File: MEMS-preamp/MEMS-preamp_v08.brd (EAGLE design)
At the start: 51 x 30 mm, 46 parts, among them IC1 DMN2400, IC2 BQ21040, IC3 BQ297X, IC4 SC4503, IC5 TPS7A49, IC6 OPA2134, J2 Battery, SW1 SPDT

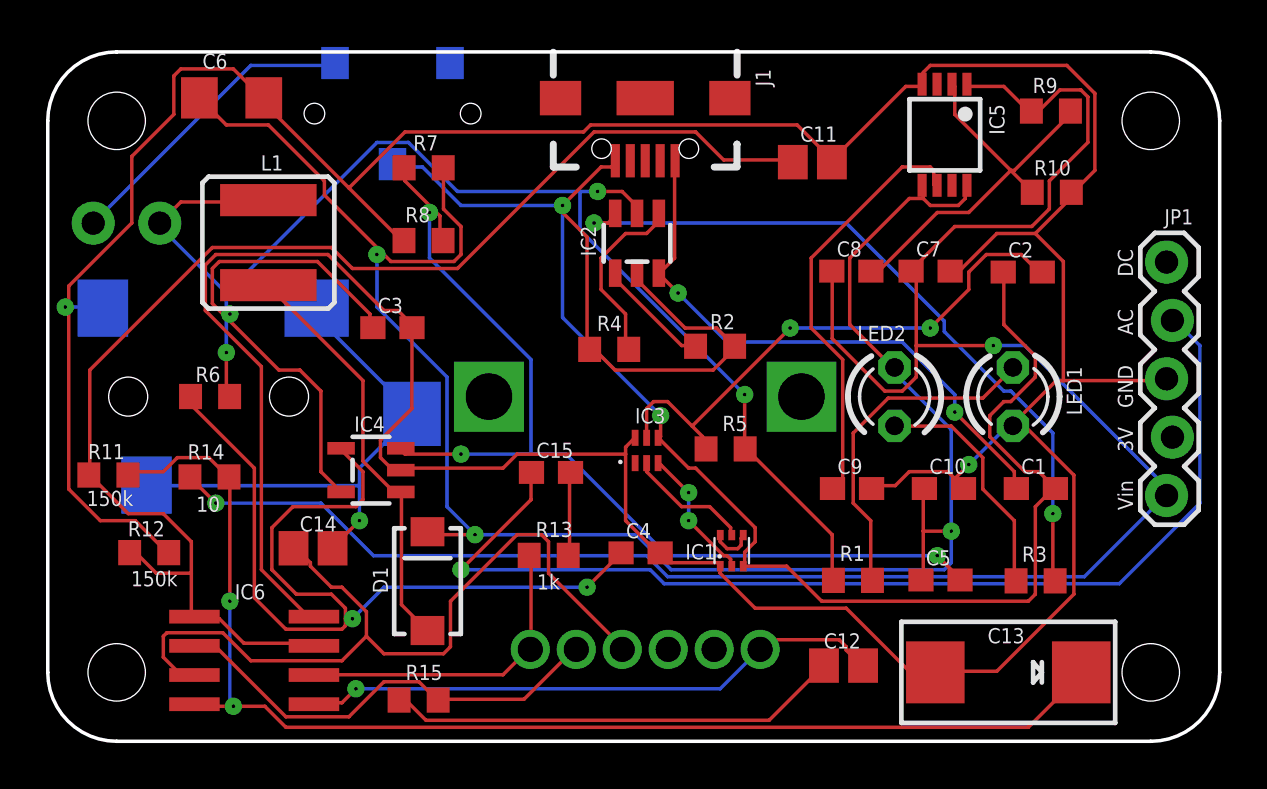
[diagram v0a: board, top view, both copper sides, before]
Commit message: Add files via upload
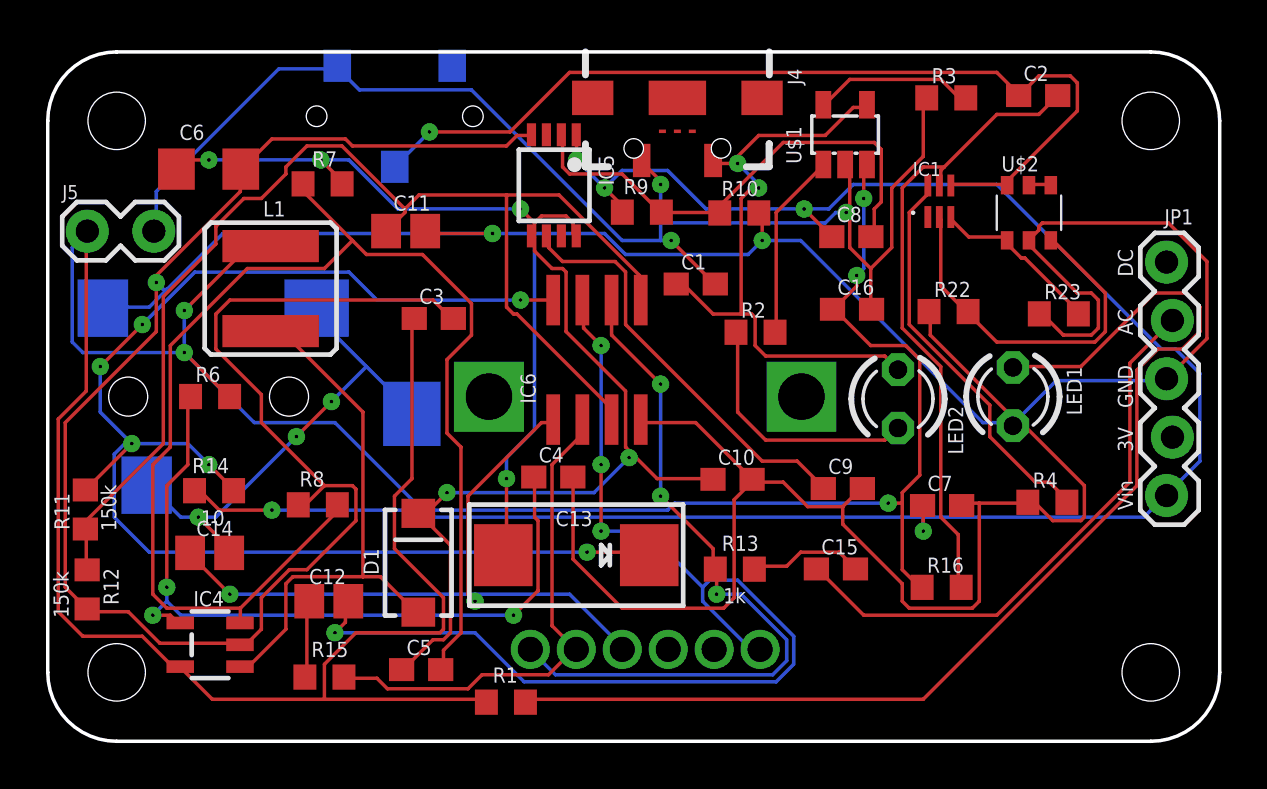
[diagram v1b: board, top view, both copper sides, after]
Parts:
- removed IC2: BQ21040, CMU-ArtFab:SOT23-6
- removed IC3: BQ297X, CMU-ArtFab:WSON-6
- removed J1: (no value), SparkFun-Connectors:USB-B-MICRO-SMD_RED_PASTE
- removed J2: Battery, SparkFun-Connectors:1X02_LOCK
- removed R5: 330, CMU-ArtFab:R0603
- removed SW1: SPDT, CMU-ArtFab:SWITCH_SPDT_CL-SB-12B
- added C16: 4.7uF, rcl:C0603
- added J4: (no value), CMU-ArtFab:USB-B-MICRO-SMD_RED_PASTE
- added J5: Battery, SparkFun-Connectors:1X02_LOCK
- added R16: 330, CMU-ArtFab:R0603
- added R22, R23: 10M, CMU-ArtFab:R0603
- added SW3: SPDT, CMU-ArtFab:SWITCH_SPDT_CL-SB-12B
- added U$1: MCP73831, CMU-ArtFab:SOT-23-5
- added U$2: QS6K1, CMU-ArtFab:SOT457R_PHILIPS
- C1: value 10uF -> 4.7uF
- IC1: value DMN2400 -> BQ297X; device CMU-ArtFab:SOT-563 -> CMU-ArtFab:WSON-6-LONG
- IC6: value OPA2134 -> TL072D
- LED2: value (none) -> Charge
- R2: value 10k -> 470
- R3: value 1k -> 5k
- R4: value 10k -> 2.2k
- moved C5 22.9 mm to (16.2, 3.12)
- moved C12 22.6 mm to (12.2, 6.09)
- moved R3 21.4 mm to (39.1, 28.0)
- moved R4 20.2 mm to (43.5, 10.4)
- moved IC6 19.8 mm to (23.9, 16.6), turned to 0 degrees
- moved C13 19.5 mm to (23.0, 8.10)
- moved R9 18.3 mm to (25.9, 23.0)
- moved C11 18.0 mm to (15.6, 22.2)
- moved IC1 17.7 mm to (38.8, 23.5)
- moved C1 17.3 mm to (28.2, 19.9)
- moved IC5 17.1 mm to (22.0, 24.2)
- moved R1 16.0 mm to (19.9, 1.70)
- moved R10 13.6 mm to (30.1, 23.0)
- moved C15 13.1 mm to (34.3, 7.50)
- moved R8 12.4 mm to (11.8, 10.3)
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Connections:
- removed net GND2: C1.2, C2.1, IC1.3, IC2.5, IC3.4, J1.GND, R2.1, R4.1, SW1.P$2
- removed net N$15: IC2.3, R3.2
- removed net N$16: IC2.1, R4.2
- removed net N$17: IC2.4, R2.2
- removed net N$18: C2.2, IC3.5, R5.2
- removed net N$19: IC1.4, IC1.6
- removed net N$20: IC1.5, IC3.2
- removed net VUSB: C1.1, IC2.6, J1.VBUS
- new net +5V: C1.1, J4.VBUS, LED2.A, U$1.4
- new net BATGND: C2.1, IC1.4, SW3.P$2, U$2.6
- new net N$25: R2.2, U$1.1
- new net N$27: IC1.3, R23.2, U$2.1
- new net N$31: IC1.2, R22.2, U$2.3
- new net N$34: IC1.6, R4.2
- new net N$42: C2.2, IC1.5, R16.2
- new net USBGND: C1.2, C16.2, J4.GND, J5.2, R3.1, SW3.P$1, U$1.2
- net GND: now also R22.1, R23.1, R4.1, U$2.2; no longer IC1.1, IC3.6
- net N$10: now also IC6.1; no longer IC6.7
- net N$11: now also U$2.4, U$2.5; no longer LED2.K, R3.1
- net N$21: now also IC6.2; no longer IC6.6
- net N$22: now also LED2.K, R2.1; no longer IC1.2, IC3.3
- net N$5: now also IC6.6; no longer IC6.2
- net N$6: now also R3.2, U$1.5; no longer J2.2, SW1.P$1
- net N$9: now also IC6.7; no longer IC6.1
- net V+: no longer LED2.A
- net VBAT: now also C16.1, J5.1, R16.1, U$1.3; no longer IC2.2, J2.1, R5.1
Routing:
- net GND2: track 81.7 -> 0.00 mm, vias 2 -> 0
- net USBGND: track 0.00 -> 59.8 mm, vias 0 -> 3
- net VBAT: track 79.0 -> 135.6 mm, vias 4 -> 5
- net BATGND: track 0.00 -> 40.6 mm, vias 0 -> 1
- net GND: track 194.6 -> 231.0 mm, vias 2 -> 4
- net N$2: track 14.9 -> 49.8 mm
- net N$15: track 31.7 -> 0.00 mm, vias 2 -> 0
- net V+: track 84.7 -> 56.2 mm, vias 3 -> 5
- net N$42: track 0.00 -> 27.8 mm
- net +5V: track 0.00 -> 27.4 mm, vias 0 -> 2
- net VUSB: track 25.5 -> 0.00 mm, vias 2 -> 0
- net N$18: track 24.2 -> 0.00 mm, vias 2 -> 0
- net N$9: track 25.6 -> 48.9 mm, vias 1 -> 4
- net N$3: track 47.9 -> 24.7 mm, vias 1 -> 0
- net N$5: track 14.0 -> 31.4 mm, vias 0 -> 3
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
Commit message: Add files via upload
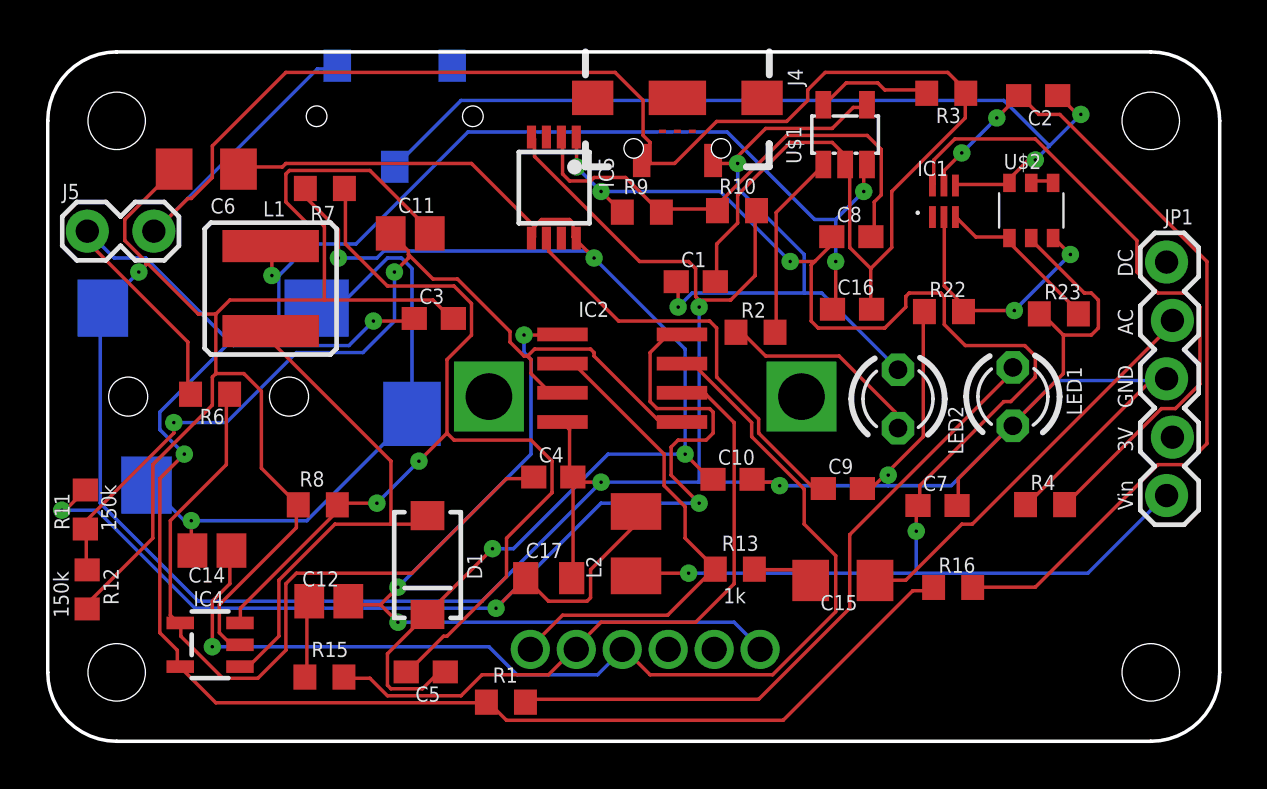
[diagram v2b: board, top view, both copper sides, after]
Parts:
- removed C13: 100uF, microbuilder:EIA7343-31/D-R
- removed IC6: TL072D, linear:SO08
- removed R14: 10, CMU-ArtFab:R0603
- added C17: 0.1uF, adafruit:C0805K
- added IC2: OPA2134UA, linear:SO08
- added L2: 100uH/500mA, rcl:L3225M
- C15: device rcl:C0603 -> rcl:C1206
- moved C15 0.58 mm to (34.6, 7.00), turned to 180 degrees
- moved R16 0.50 mm to (39.4, 6.70)
- moved D1 0.41 mm to (16.5, 7.67), turned to 270 degrees
- moved R7 0.22 mm to (12.1, 24.1), turned to 180 degrees
- moved C11 0.22 mm to (15.8, 22.1)
- moved C5 0.22 mm to (16.4, 3.02), turned to 180 degrees
- moved C7 0.20 mm to (38.7, 10.3)
- moved IC1 0.20 mm to (39.0, 23.5)
- moved R22 0.20 mm to (39.0, 18.7)
- moved R3 0.20 mm to (39.1, 28.2), turned to 180 degrees
- moved C14 0.14 mm to (7.14, 8.30), turned to 180 degrees
- moved R4 0.14 mm to (43.4, 10.3)
- moved R10 0.14 mm to (30.0, 23.1)
- moved U$2 0.14 mm to (42.8, 23.1)
- moved C1 0.10 mm to (28.2, 20.0)
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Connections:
- removed net N$1: C13.+, IC6.8, R11.2, R14.1
- new net N$15: C17.1, IC2.8, L2.2, R11.2
- net +12V: now also L2.1; no longer R14.2
- net GND: now also C17.2, IC2.4; no longer C13.-, IC6.4
- net N$10: now also IC2.7; no longer IC6.1
- net N$21: now also IC2.6; no longer IC6.2
- net N$5: now also IC2.2; no longer IC6.6
- net N$8: now also IC2.3, IC2.5; no longer IC6.3, IC6.5
- net N$9: now also IC2.1; no longer IC6.7
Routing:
- net N$1: track 61.6 -> 0.00 mm, vias 6 -> 0
- net N$15: track 0.00 -> 55.3 mm, vias 0 -> 3
- net GND: track 231.0 -> 199.7 mm, vias 4 -> 5
- net USBGND: track 59.8 -> 82.8 mm, vias 3 -> 0
- net N$2: track 49.8 -> 29.3 mm
- net +12V: track 87.6 -> 67.8 mm
- net N$10: track 30.8 -> 48.1 mm, vias 2 -> 1
- net VBAT: track 135.6 -> 118.5 mm
- net N$9: track 48.9 -> 35.1 mm, vias 4 -> 3
- net N$14: track 58.6 -> 45.0 mm, vias 0 -> 2
- net N$8: track 54.5 -> 42.0 mm, vias 0 -> 2
- net N$34: track 17.3 -> 28.3 mm
- net V+: track 56.2 -> 66.2 mm, vias 5 -> 4
- net N$5: track 31.4 -> 21.6 mm, vias 3 -> 0
- net N$42: track 27.8 -> 37.1 mm, vias 0 -> 2
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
